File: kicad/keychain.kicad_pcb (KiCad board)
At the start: 2 copper layers, 68 x 38 mm, 19 parts, among them J1 EPAPER, J2 SuperMini-L, J3 SuperMini-R, J4 BATTERY, SW1 SW_SPDT, U1 TP4056

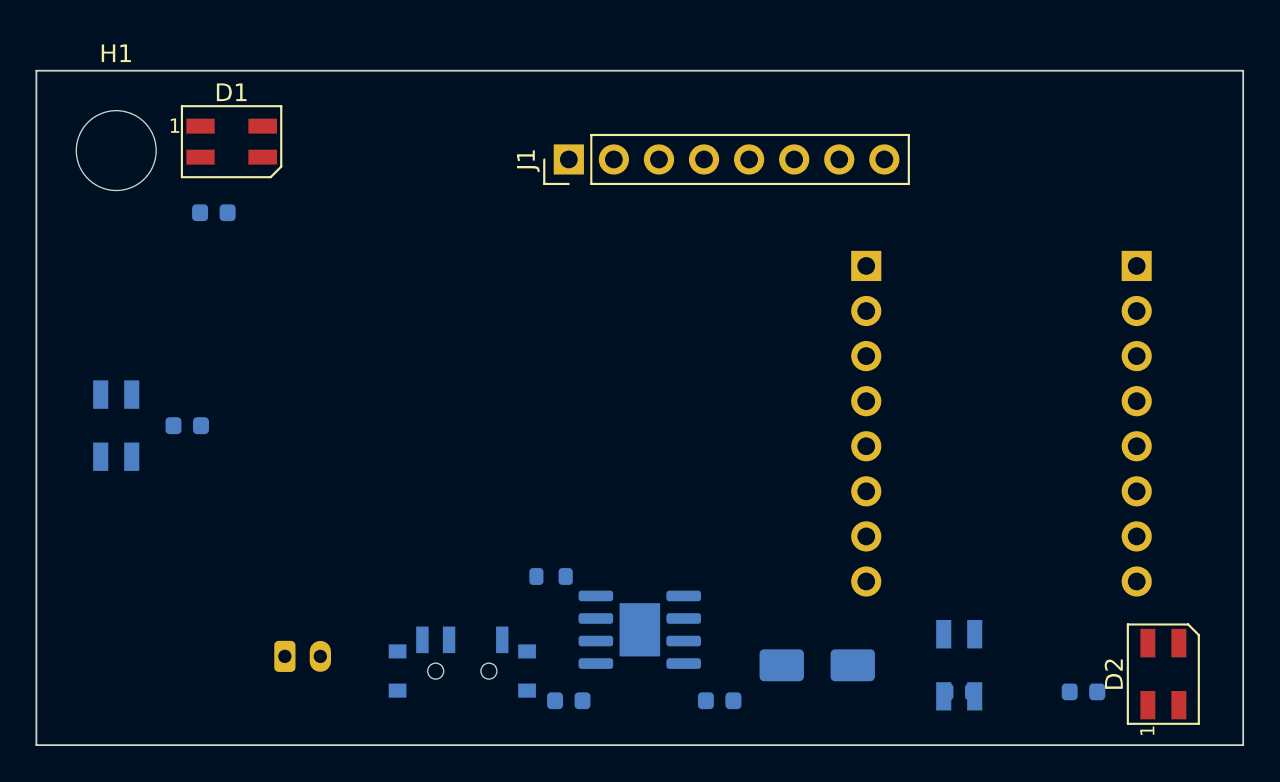
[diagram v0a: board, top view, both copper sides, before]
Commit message: Route board: A* router, 0 unconnected (0.3mm sig/0.5mm pwr, vias, GND zones)
Generated with [Devin](https://devin.ai)

Co-Authored-By: Devin <158243242+devin-ai-integration[bot]@users.noreply.github.com>
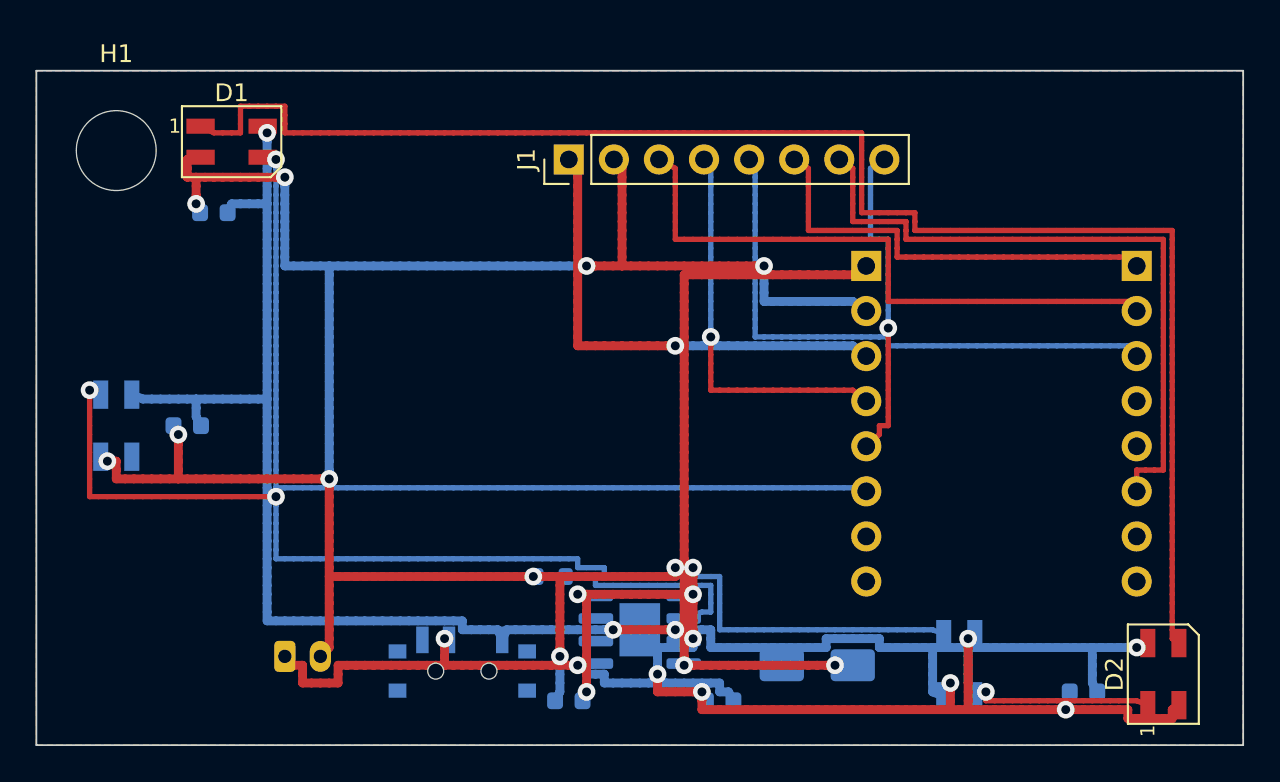
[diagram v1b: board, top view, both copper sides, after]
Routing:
- net GND: track 0.00 -> 175.9 mm, vias 0 -> 18
- net VBAT_SW: track 0.00 -> 103.8 mm, vias 0 -> 4
- net D1_DO: track 0.00 -> 86.8 mm
- net D3_DO: track 0.00 -> 62.3 mm, vias 0 -> 2
- net +5V: track 0.00 -> 55.1 mm, vias 0 -> 4
- net LED_DATA: track 0.00 -> 52.5 mm, vias 0 -> 1
- net EPD_RST: track 0.00 -> 38.1 mm
- net EPD_MOSI: track 0.00 -> 34.8 mm
- net VBAT: track 0.00 -> 33.1 mm, vias 0 -> 2
- net EPD_CS: track 0.00 -> 32.4 mm
- net +3.3V: track 0.00 -> 27.2 mm, vias 0 -> 1
- net EPD_DC: track 0.00 -> 24.7 mm
- net EPD_CLK: track 0.00 -> 22.1 mm, vias 0 -> 1
- net EPD_BUSY: track 0.00 -> 18.4 mm, vias 0 -> 1
- net PROG: track 0.00 -> 11.8 mm
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- added copper zone on B.Cu, net GND
- added copper zone on F.Cu, net GND
